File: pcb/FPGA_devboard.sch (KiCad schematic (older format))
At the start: 2 parts, among them X5 Conn_02x05_Odd_Even, X6 AC7020

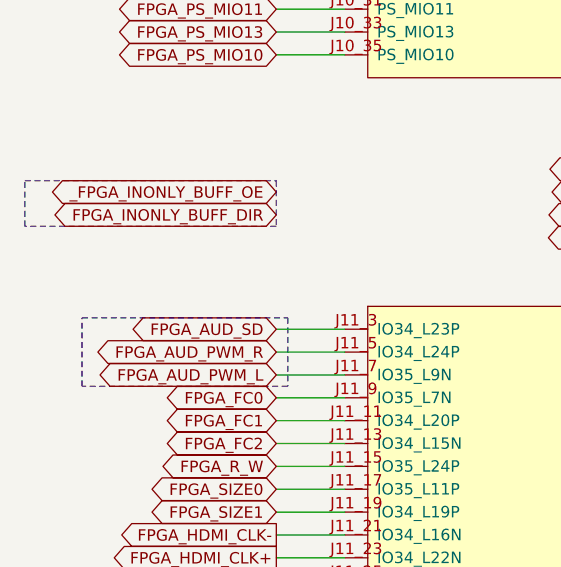
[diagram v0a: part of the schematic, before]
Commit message: pinout changes
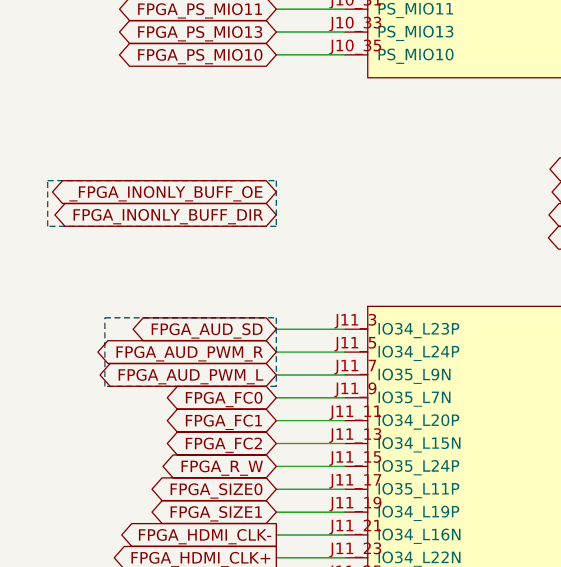
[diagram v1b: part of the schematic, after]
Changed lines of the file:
@@
 	4600 3200 4300 3200
 Wire Notes Line
-	950  4650 950  4350
+	1050 4650 1050 4350
 Wire Notes Line
-	950  4350 1850 4350
+	1050 4350 1800 4350
 Wire Notes Line
-	1850 4650 950  4650
+	1800 4650 1050 4650
 Wire Notes Line
 	5300 5450 4650 5450
@@
 	1800 3750 1800 3950
 Wire Notes Line
-	700  3950 700  3750
+	800  3950 800  3750
 Wire Notes Line
 	4600 3050 5250 3050
@@
 FPGA_HDMI_CLK+
 Wire Notes Line
-	1800 3950 700  3950
+	1800 3950 800  3950
 Wire Notes Line
-	700  3750 1800 3750
+	800  3750 1800 3750
 Text GLabel 4600 5800 2    50   BiDi ~ 0
 _FPGA_DS
@@
 _FPGA_INONLY_BUFF_OE
 Wire Notes Line
-	1850 4350 1850 4650
+	1800 4350 1800 4650
 Text GLabel 1800 5300 0    50   Output ~ 0
 FPGA_HDMI_CLK-
